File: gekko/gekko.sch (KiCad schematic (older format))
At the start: 81 parts, among them J10 Conn_01x02, J11 Conn_01x02, J3 Conn_01x05, J4 Conn_01x03, J6 Conn_01x02, Q1 Q_NMOS_GSD, SW1 SW_Push_Dual_x2, SW2 SW_DPDT_x2, U1 DRV8835, U12 sw_pch, U2 STM32F413CH6, U3 LED_FOTR, U4 LP5907_DBV, U5 ICM20648, U6 LED_FOTR, U7 LED_FOTR, U8 LED_FOTR, U9 RP124N334E-TR-FE, Y1 Crystal_GND23

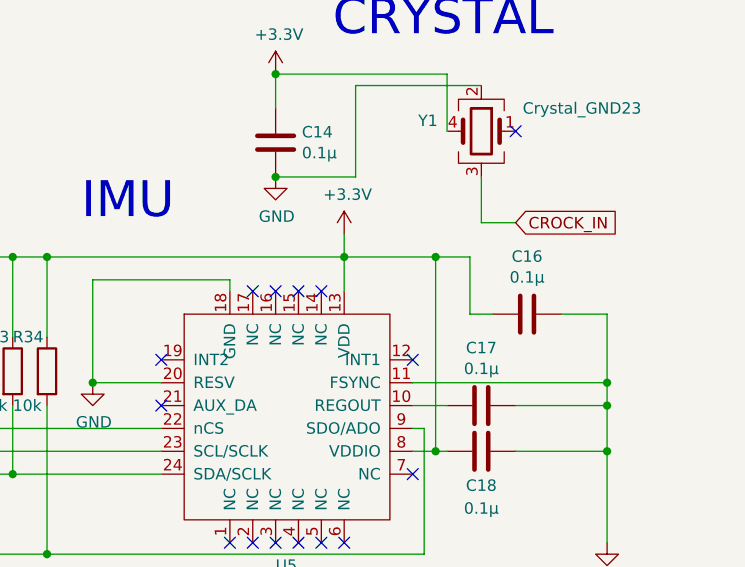
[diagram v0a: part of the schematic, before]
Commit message: RE_patern_finish
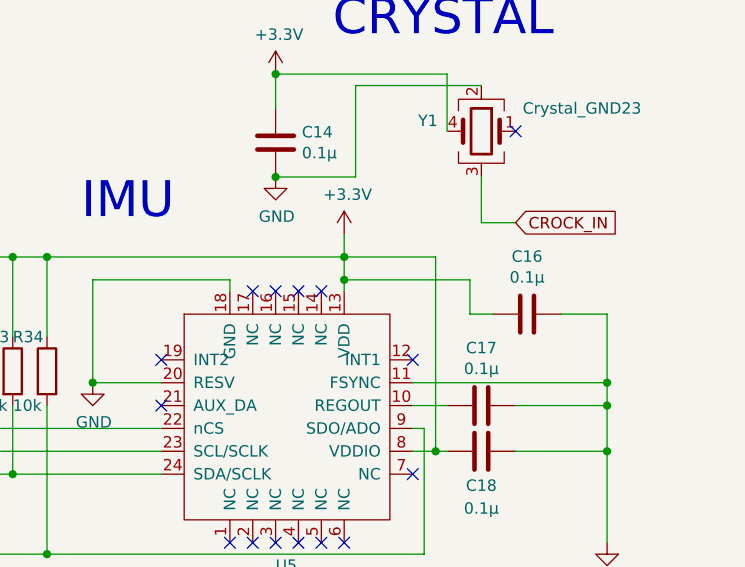
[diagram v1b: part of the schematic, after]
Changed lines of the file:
@@
 Connection ~ 9600 5050
 Wire Wire Line
-	9600 5050 9600 5200
+	9600 5050 9600 5150
 NoConn ~ 9900 5500
 Wire Wire Line
@@
 	10550 5300 10750 5300
 Wire Wire Line
-	10150 5050 10150 5300
-Wire Wire Line
 	9600 5050 10000 5050
 Wire Wire Line
@@
 Wire Wire Line
 	10000 5900 10050 5900
-Connection ~ 10000 5050
-Wire Wire Line
-	10000 5050 10150 5050
 Text GLabel 5500 5100 3    50   Input ~ 0
 battery_wt
@@
 Text GLabel 5050 4600 0    50   Input ~ 0
 MotorL_Reverce
+Wire Wire Line
+	9600 5150 10150 5150
+Wire Wire Line
+	10150 5150 10150 5300
+Connection ~ 9600 5150
+Wire Wire Line
+	9600 5150 9600 5200
 $EndSCHEMATC
